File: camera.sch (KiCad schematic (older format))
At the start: 37 parts, among them P10 CONN_01X14, P11 CONN_01X12, Q1 2SC5095, Q2 MT3S20TU, Q3 2SC5095, Q4 MT3S20TU, U10 ICX825AQA, U9 CXD3400N

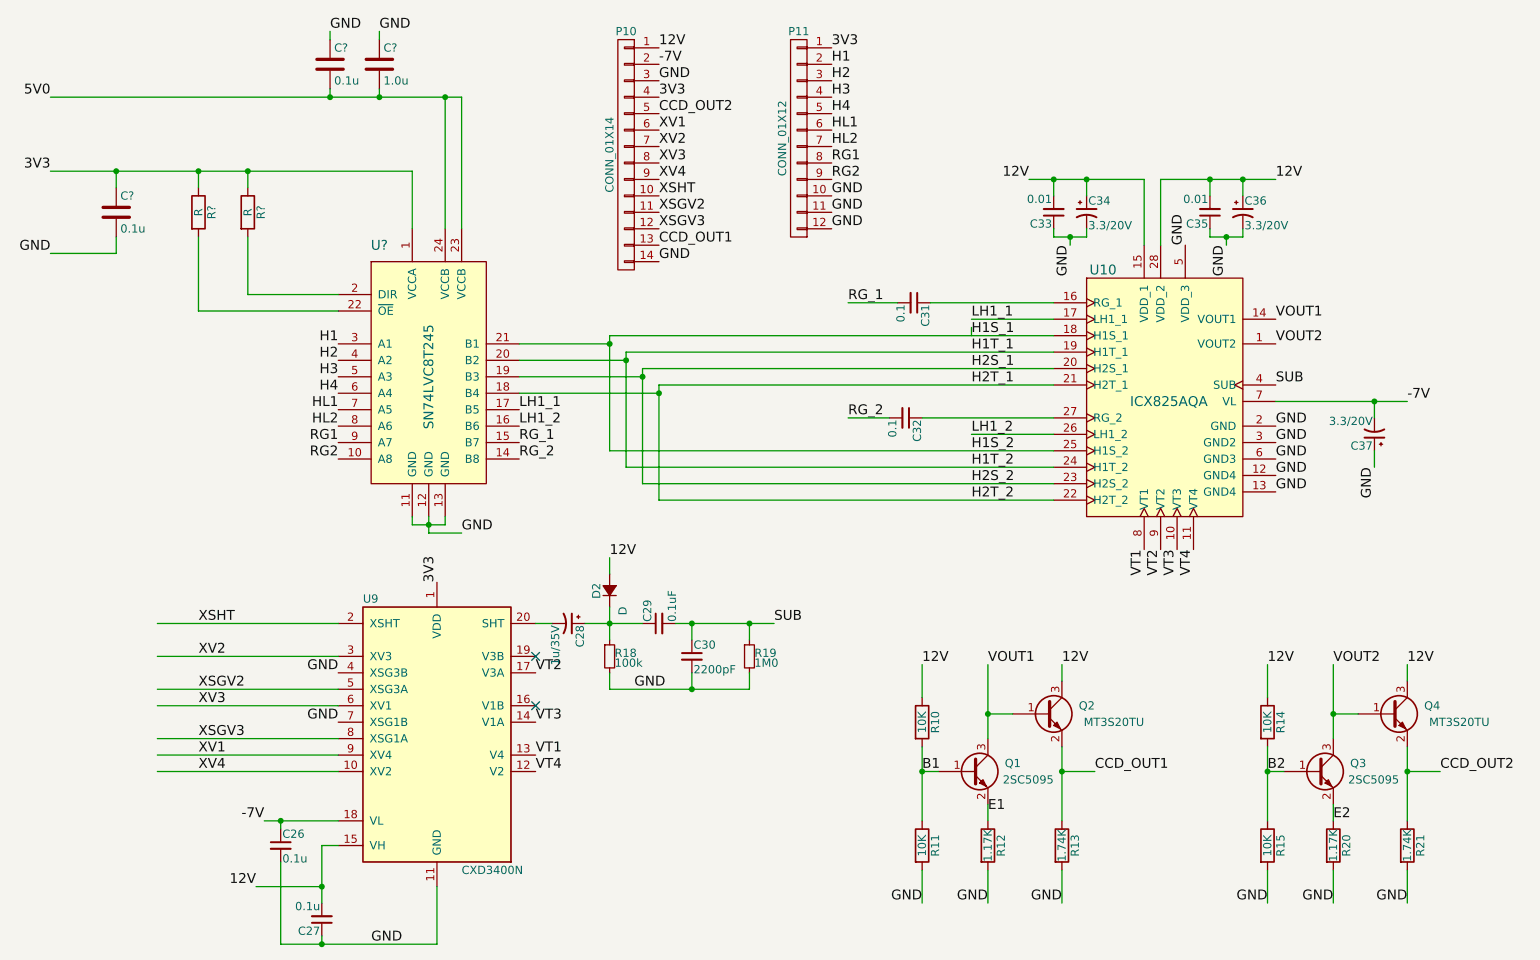
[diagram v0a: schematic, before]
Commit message: lots of work
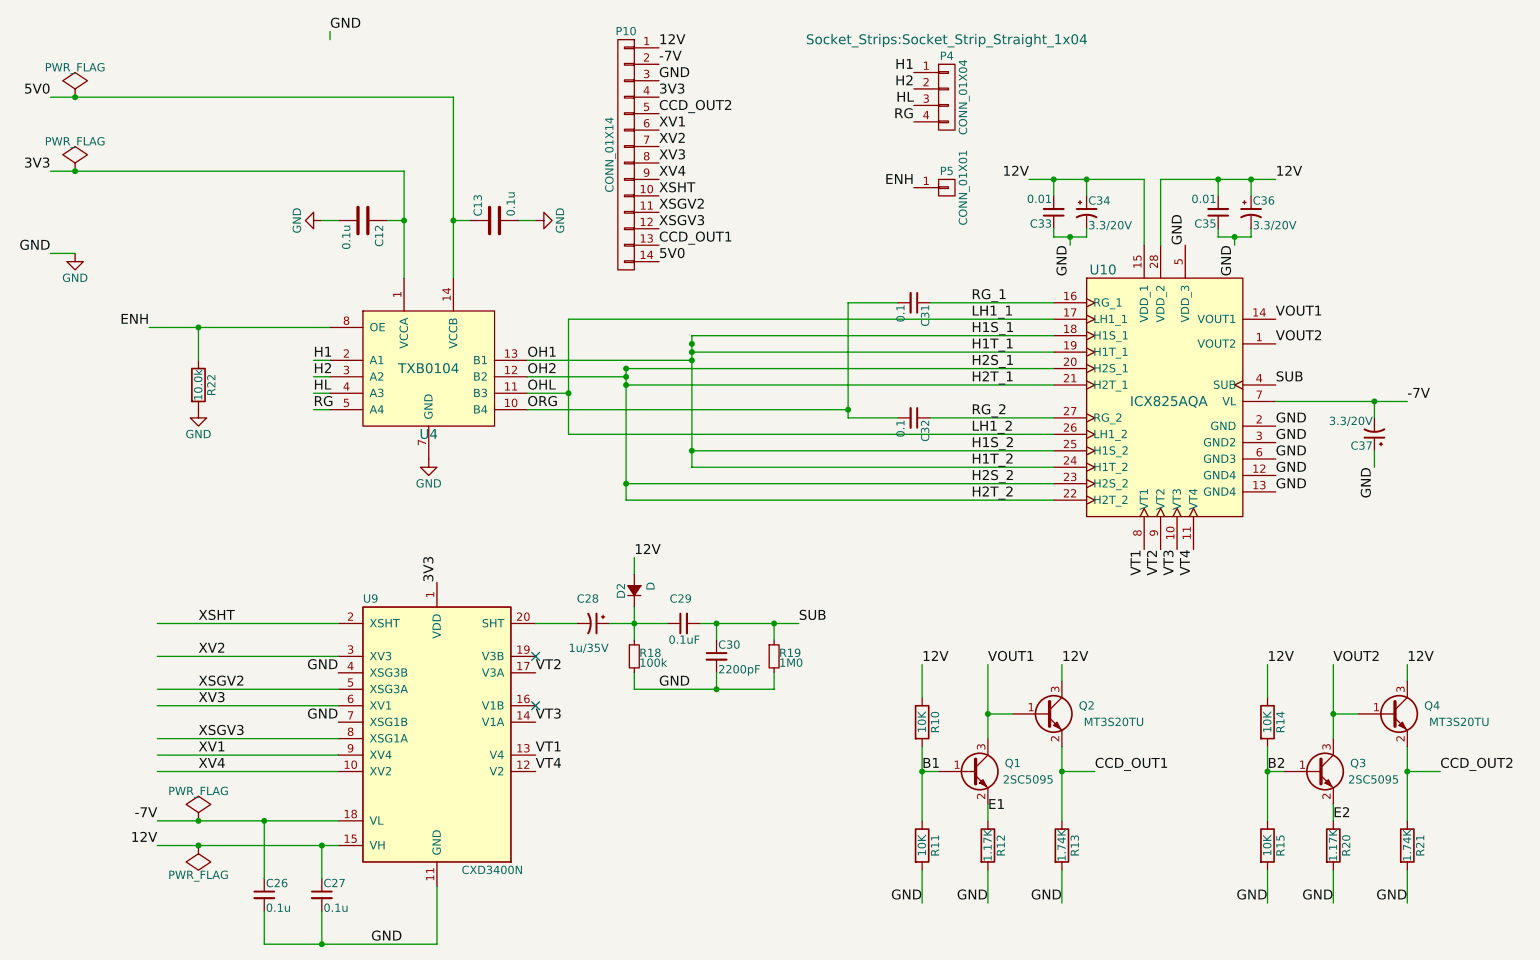
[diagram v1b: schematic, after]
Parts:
- removed C?: 1.0u, symbol C
- removed P11: CONN_01X12, w_pin_strip:pin_strip_12, symbol CONN_01X12
- removed R?: R, symbol R
- removed U?: SN74LVC8T245, symbol SN74LVC8T245
- added P4: CONN_01X04, Socket_Strips:Socket_Strip_Straight_1x04, symbol CONN_01X04
- added P5: CONN_01X01, Socket_Strips:Socket_Strip_Straight_1x01, symbol CONN_01X01
- added U4: TXB0104, Housings_SSOP:TSSOP-14_4.4x5mm_Pitch0.65mm, symbol TXB0104
- C12, C13: renamed from C?; footprint (none) -> Capacitors_SMD:C_0603
- C26, C27, C29, C30, C31, C32, C33: footprint w_smd_cap:c_0603 -> Capacitors_SMD:C_0603
- C28, C34, C36, C37: footprint w_smd_cap:c_0805 -> Capacitors_SMD:c_elec_4x5.3
- C35: footprint w_smd_cap:c_0805 -> Capacitors_SMD:C_0603
- D2: footprint w_smd_diode:sod123 -> Diodes_SMD:SOD-123
- P10: footprint w_pin_strip:pin_strip_14 -> Pin_Headers:Pin_Header_Straight_1x14
- R10, R11, R12, R13, R14, R15, R18, R19, R20, R21: footprint w_smd_resistors:r_0805 -> Resistors_SMD:R_0603_HandSoldering
- R22: renamed from R?; value R -> 10.0k; footprint (none) -> Resistors_SMD:R_0603_HandSoldering
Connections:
- net labels added: ENH, HL, OH1, OH2, OHL, ORG, RG
- net labels removed: H3, H4, HL1, HL2, RG1, RG2
- wire segments 149 -> 107
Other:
- moved on the sheet: C12, C13, C26, C27, C28, C29, C30, C32, C35, C36, D2, R18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
